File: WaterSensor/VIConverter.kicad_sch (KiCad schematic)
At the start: 14 parts, among them U1 ${SIM.PARAMS}, U11 ${SIM.PARAMS}, U12 ${SIM.PARAMS}, U2 ${SIM.PARAMS}

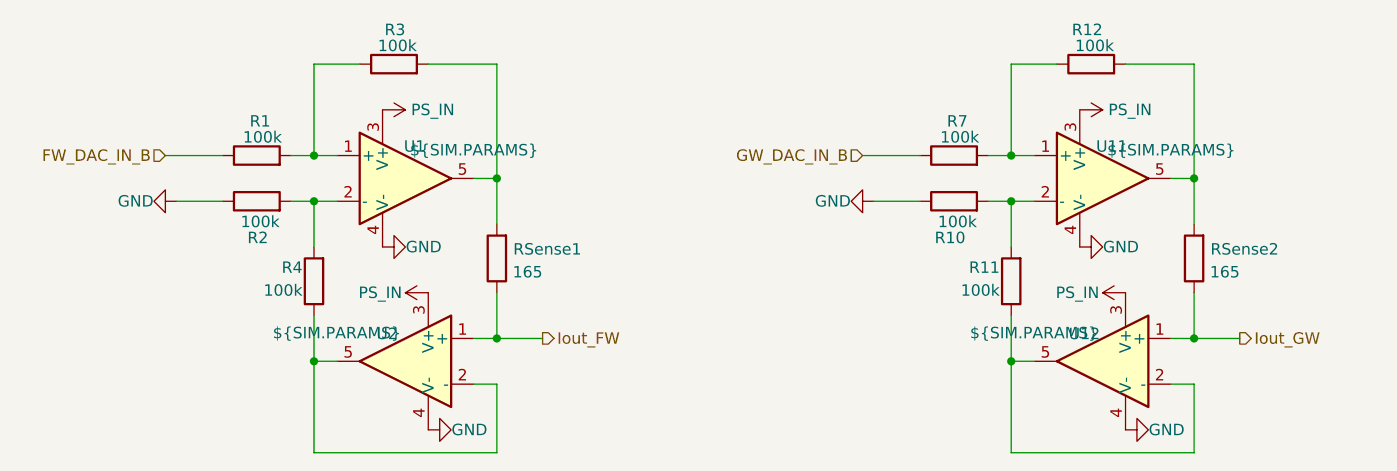
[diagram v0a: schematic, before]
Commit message: ready to manufacture
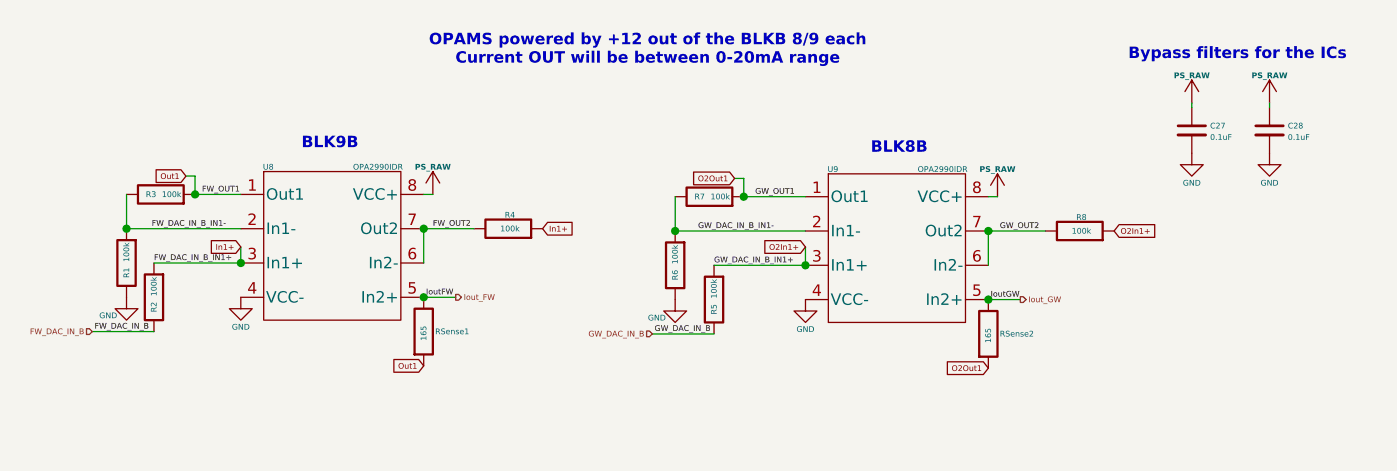
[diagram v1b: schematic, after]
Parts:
- removed R10, R11, R12: 100k, symbol Device:R
- removed U1, U11, U12, U2: ${SIM.PARAMS}, symbol Simulation_SPICE:OPAMP
- added C27, C28: 0.1uF, Capacitor_SMD:C_0603_1608Metric, symbol Device:C_Small
- added R5, R6, R8: 100k, Resistor_SMD:R_0603_1608Metric, symbol Device:R
- added U8, U9: OPA2990IDR, OPA2990IDR:D8_TEX-M, symbol TSV632:TSV632
- R1, R2, R3, R4, R7, RSense1, RSense2: footprint (none) -> Resistor_SMD:R_0603_1608Metric
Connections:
- net FW_DAC_IN_B: now also R2.1; no longer R1.1
- net GND: now also R1.1, C27.2, C28.2, R6.1, U8.4 (VCC-), U9.4 (VCC-); no longer R2.1
- net GW_DAC_IN_B: now also R5.1; no longer R7.1
- net Iout_FW: now also U8.5 (In2+)
- net Iout_GW: now also U9.5 (In2+)
- net Out1: now reaches R3.2, RSense1.2
- net Out1: now also U8.1 (Out1)
- net O2Out1: now reaches R7.2
- net O2Out1: now also RSense2.2, U9.1 (Out1)
- net In1+: now reaches R2.2, R4.2
- net In1+: now also U8.3 (In1+)
- net FW_OUT2: now reaches R4.1
- net FW_OUT2: now also U8.6 (In2-), U8.7 (Out2)
- net FW_DAC_IN_B_IN1-: now reaches R1.2, R3.1
- net FW_DAC_IN_B_IN1-: now also U8.2 (In1-)
- new net GW_DAC_IN_B_IN1-: R6.2, R7.1, U9.2 (In1-)
- new net GW_OUT2: R8.1, U9.6 (In2-), U9.7 (Out2)
- new net O2In1+: R5.2, R8.2, U9.3 (In1+)
- new net PS_RAW: C27.1, C28.1, U8.8 (VCC+), U9.8 (VCC+)
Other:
- note added: "BLK8B"
- note added: "BLK9B"
- note added: "Bypass filters for the ICs"
- note added: "OPAMS powered by +12 out of the BLKB 8/9 each Current OUT will be between 0-20mA range"
